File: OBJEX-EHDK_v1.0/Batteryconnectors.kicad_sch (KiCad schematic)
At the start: 19 parts, among them J1 Conn_LiPoBattery, J2 JST_SM02B, J3 SELECT BATT CONN, Q1 NTNUS3171PZT5G

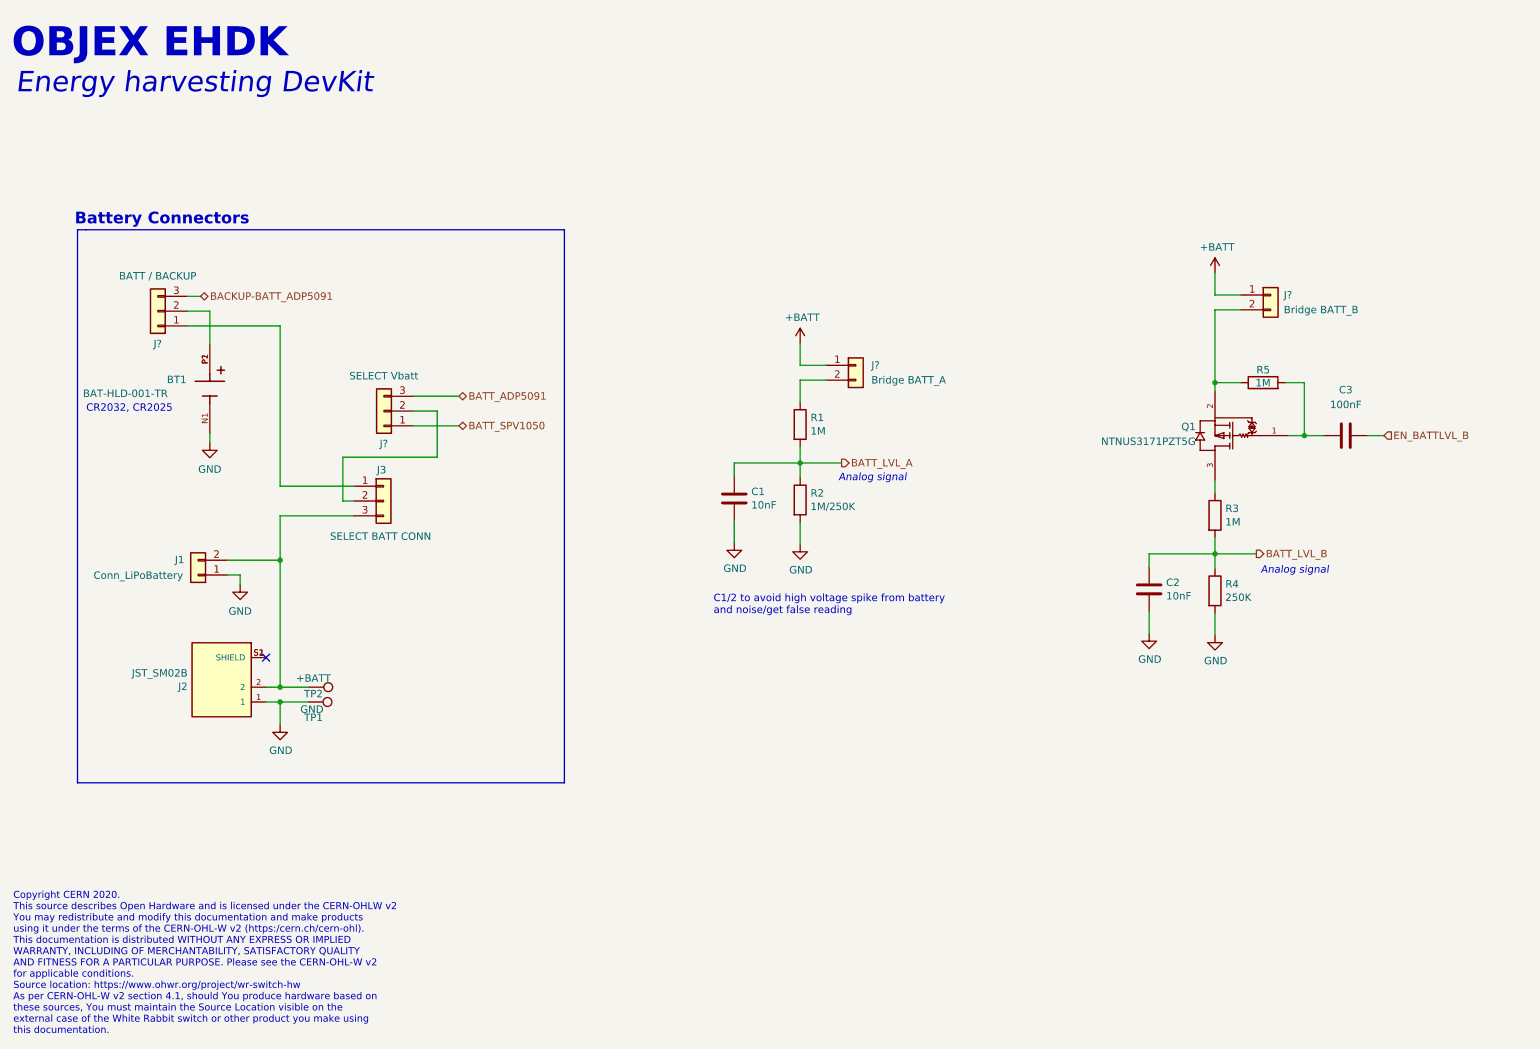
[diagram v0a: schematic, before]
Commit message: update
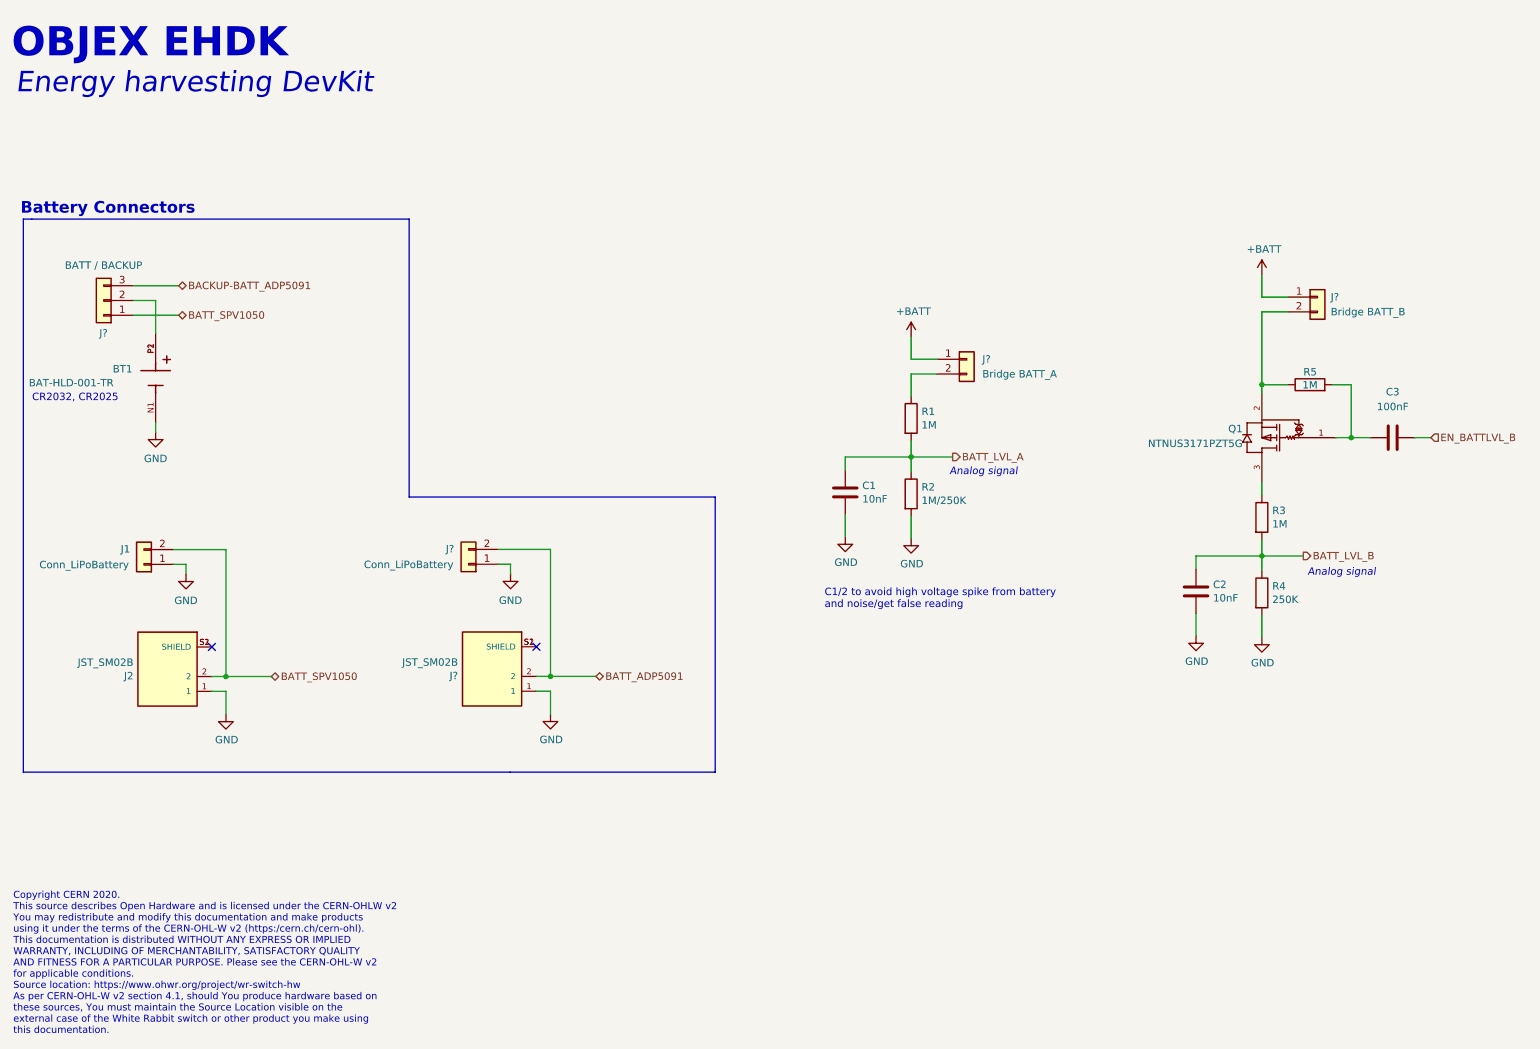
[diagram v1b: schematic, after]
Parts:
- removed J3: SELECT BATT CONN, symbol Connector_Generic:Conn_01x03
- removed J?: SELECT Vbatt, symbol Connector_Generic:Conn_01x03
- removed TP1: GND, TestPoint:TestPoint_Pad_1.5x1.5mm, symbol Connector:TestPoint
- removed TP2: +BATT, TestPoint:TestPoint_Pad_1.5x1.5mm, symbol Connector:TestPoint
- added J?: Conn_LiPoBattery, symbol Connector_Generic:Conn_01x02
- added J?: JST_SM02B, KicadLibrary:JST_SM02B-SURS-TF(LF)(SN), symbol SM02B-SURS-TF_LF__SN_:SM02B-SURS-TF(LF)(SN)
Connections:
- net BATT_ADP5091: now also J?.2, J?.2 (Pin_2)
- net BATT_SPV1050: now also J1.2 (Pin_2), J2.2, J?.1 (Pin_1)
- net GND: now also J?.1, J?.1 (Pin_1)
- new net: J?.S1 (SHIELD), J?.S2 (SHIELD)
- no-connect marks 1 -> 2
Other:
- moved on the sheet: BT1, C1, C2, C3, J1, J2, J?, Q1, R1, R2, R3, R4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
